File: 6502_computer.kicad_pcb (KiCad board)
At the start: 4 copper layers, 169.5 x 112.1 mm, 19 parts, among them J1 Barrel_Jack_Switch, J2 Conn_01x16, J3 Mega, J4 Mega, J5 Clock, J6 Conn_01x40, J7 Conn_01x06, J8 Conn_01x02, J9 Conn_01x02, U1 6502_mainboard_v2, U2 W65C22SxP, U3 Keyboard_v1

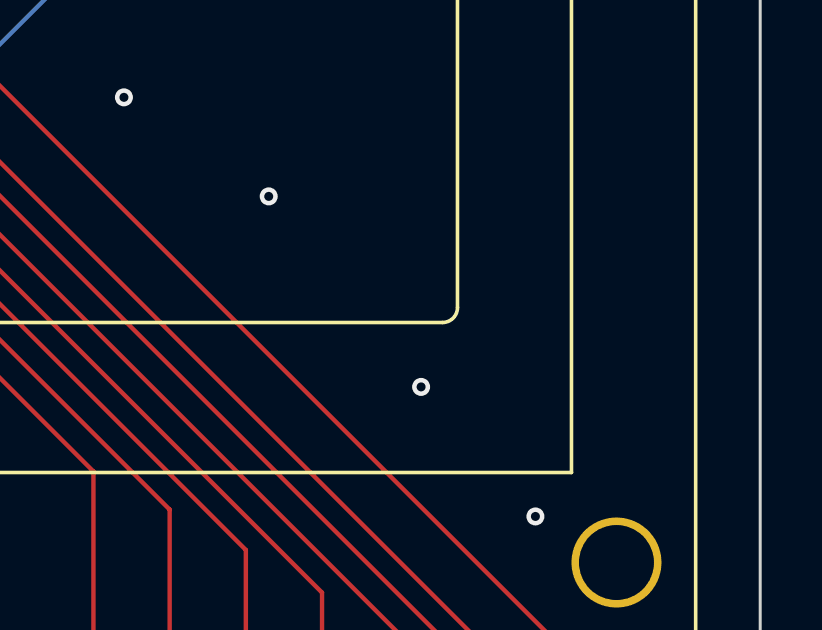
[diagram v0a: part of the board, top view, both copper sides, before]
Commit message: Update
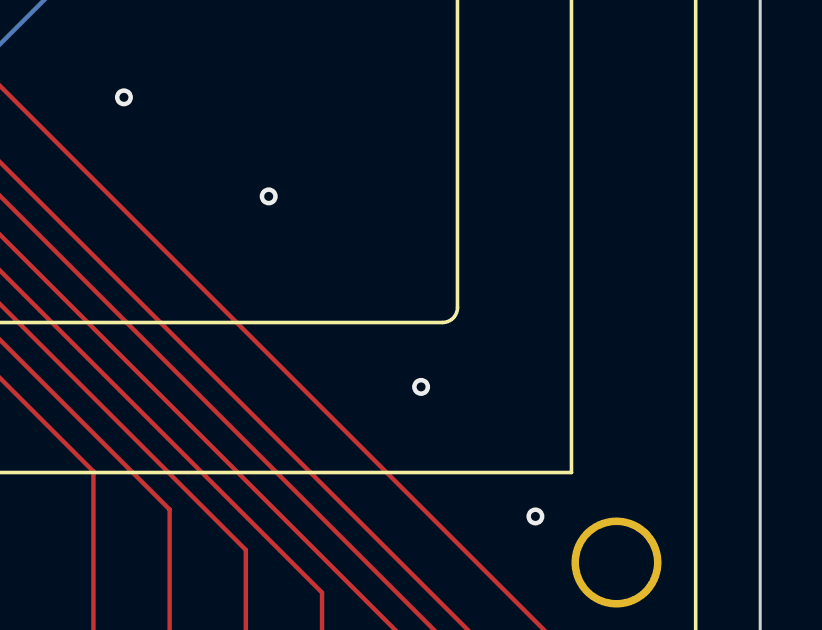
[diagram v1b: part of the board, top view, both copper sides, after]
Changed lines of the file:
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@@
     (fp_line (start 68 3) (end 68 28) (layer "F.SilkS") (width 0.12))
     (fp_arc (start -0.29972 8.49884) (mid -0.153162 8.145018) (end 0.20066 7.99846) (layer "F.SilkS") (width 0.12))
-    (fp_arc (start 64.20104 22.49932) (mid 64.054479 22.85315) (end 63.70066 22.9997) (layer "F.SilkS") (width 0.12))
+    (fp_arc (start 64.20104 22.49932) (mid 64.054473 22.853115) (end 63.70066 22.9997) (layer "F.SilkS") (width 0.12))
     (fp_arc (start 0.20066 22.9997) (mid -0.153162 22.853142) (end -0.29972 22.49932) (layer "F.SilkS") (width 0.12))
     (fp_arc (start 63.7 8) (mid 64.053553 8.146447) (end 64.2 8.5) (layer "F.SilkS") (width 0.12))
